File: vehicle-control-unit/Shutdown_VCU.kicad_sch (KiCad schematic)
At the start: 54 parts, among them K2 G6SK-2G, K3 G6DN-1A, SW1 61-6441.4047, SW2 A165E-S, SW3 Typ- 505, U10 SN74HCS08DR, U11 MCP6004, U12 SN74HCS32DR, U13 SN74HC14DR, U14 SZNUD3124DMT1G, U3 HASS-300S, U4 X05PSA02000P18, U5 X05PSA02000P18, U6 MCP6004, U7 MCP6004, U8 MCP6004, U9 SN74HCS32DR

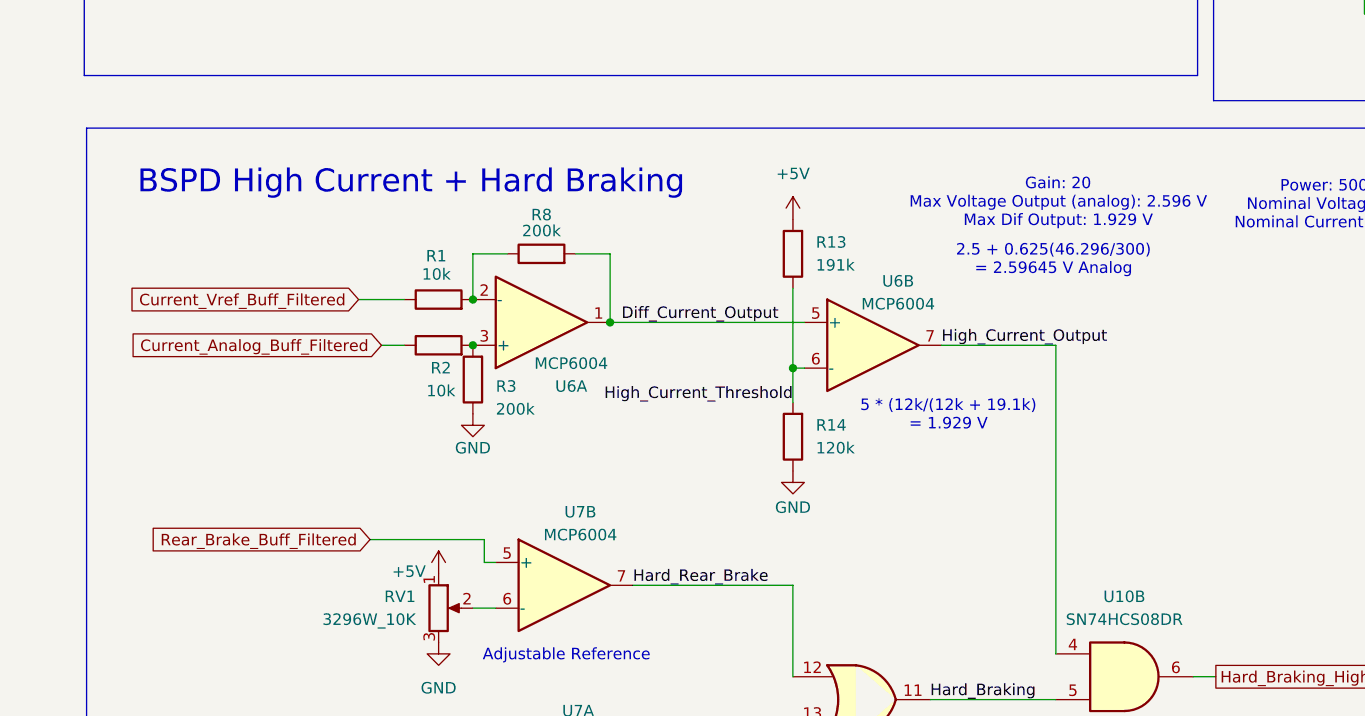
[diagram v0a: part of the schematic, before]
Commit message: added pot to BSPD current threshold
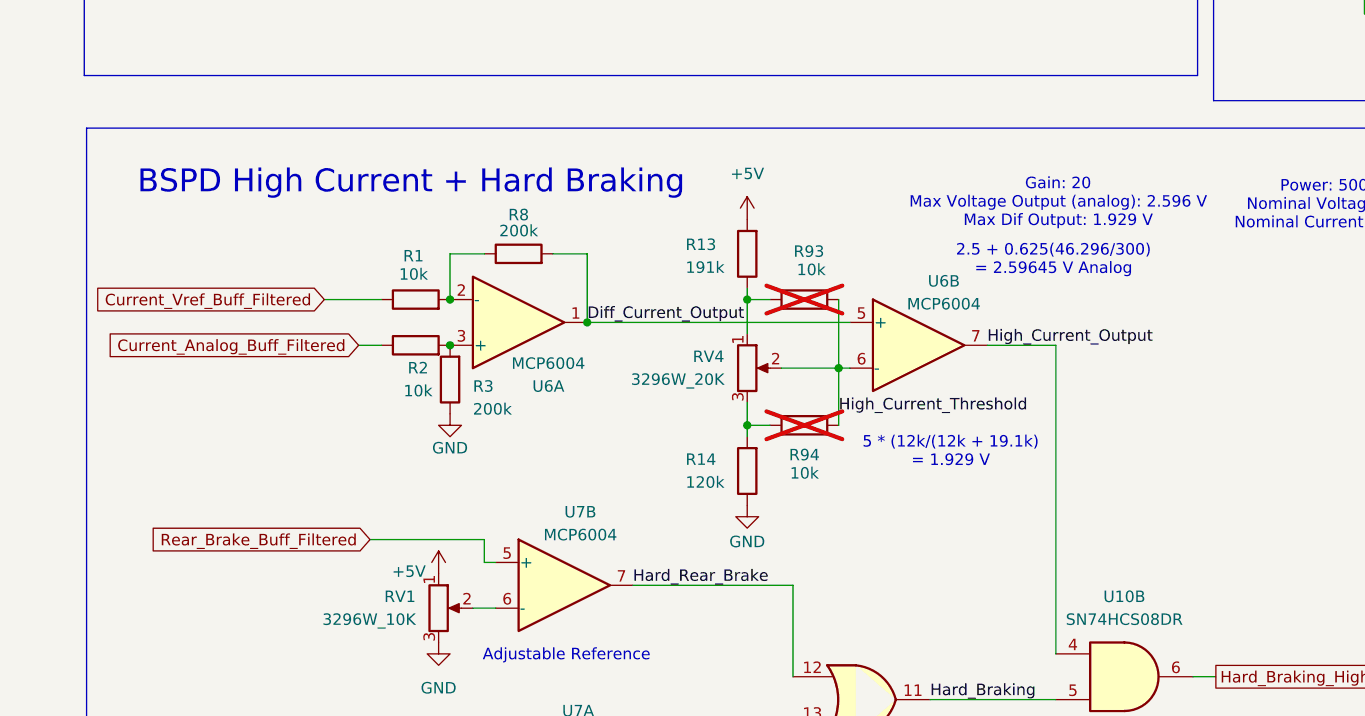
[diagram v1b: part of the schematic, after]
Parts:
- added R93, R94: 10k, Resistor_SMD:R_0603_1608Metric_Pad0.98x0.95mm_HandSolder, symbol Device:R
- added RV4: 3296W_20K, Potentiometer_THT:Potentiometer_Bourns_3296W_Vertical, symbol Device:R_Potentiometer
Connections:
- net High_Current_Threshold: now also R93.1, R94.1, RV4.2; no longer R13.1, R14.2
- new net: R13.1, R93.2, RV4.1
- new net: R14.2, R94.2, RV4.3
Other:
- moved on the sheet: R1, R13, R14, R2, R3, R8, U6A, U6B
